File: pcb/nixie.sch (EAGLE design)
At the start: 158 parts, among them IC1 STM32F100CXC, IC12 MAX603, IC2 74141N, IC3 DS3234, IC4 MAX1771, IC6 74HCT164D, IC7 DS18B20, IC8 MAX603, Q1 BUZ11BH, Q9 BSS123, X2 MINI-USB_4P-85-32004-10X

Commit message: almost done
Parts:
- removed S6: (no value), SparkFun:TAC_SWITCHPTH
- added S1, S3: (no value), Mine:TAC_SWITCH
- C1, C10, C11, C12, C13, C14, C15, C18, C20, C21, C22, C25, C26, C27, C35, C36, C4, C52, C53, C7, C8, C9, C93: value (none) -> 100n
- C16, C17, C28, C29, C92: value (none) -> 10u
- C2, C23, C3, C34, C5, Q3, R12, R51, R9: value (none) -> nc
- C24: value (none) -> 100n; device rcl:C-EUC1206 -> rcl:C-EUC0603
- C50, C51: value (none) -> 1u
- C54, L1: value (none) -> 100u
- C6: value (none) -> 2.2u 250V
- D10, D11, D8, D9: value CGRM4001-G -> (none); device diode:CGRM4001-G -> diode:DIODE-SOD123
- D2, D3, D4, D5, D6, D7: value CGRM4001-G -> 1n4148
- R1, R36, R37, R50, R6: value (none) -> 10k
- R13, R8: value (none) -> 22k
- R14, R16, R18, R20, R22, R24: value (none) -> 1M
- R15, R17, R19, R21, R23, R25: value (none) -> 47k
- R2: value (none) -> 100
- R3: value (none) -> 1k
- R30, R31: value (none) -> tbc
- R38: value (none) -> 220k
- R39, R40, R41: value (none) -> 200k
- R4: value (none) -> 0.05
- R5: value (none) -> 1M5
- R7: value (none) -> 4k7 trim
- S2, S4, S5: device SparkFun:TAC_SWITCHPTH -> Mine:TAC_SWITCH
- T1, T11, T13, T14, T3, T5, T7, T9: value (none) -> pnphv
- T10, T12, T2, T4, T6, T8: value (none) -> npnhvsmd
- T21, T22: value (none) -> npnhvth
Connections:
- net +3V3: now also S3.1; no longer S2.2, S4.2, S5.2, S6.1, S6.2
- net BUT0: now also S5.2; no longer S5.3, S5.4
- net BUT1: now also S2.2; no longer S6.3, S6.4
- net BUT2: now also S4.2; no longer S4.3, S4.4
- net BUT3: now also S3.2; no longer S2.3, S2.4
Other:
- note added: "nc"
- note added: "tbc"

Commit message: deleted stuff for merging
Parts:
- removed C23: nc, rcl:C-EUC0603
- removed C93: 100n, rcl:C-EUC0603
- removed L2: (no value), wuerth-elektronik:WE-CBF_0805
- removed R9: nc, rcl:R-EU_R0805
- removed S1: (no value), Mine:TAC_SWITCH
- removed SV6: (no value), Mine:FE06-1ED
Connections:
- removed net RXD: SV6.2
- removed net TXD: SV6.3
- net GND: no longer C93.1
- net VBAT: no longer C93.2
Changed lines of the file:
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@@
 <part name="Q3" library="crystal" deviceset="CRYSTAL" device="CTS406" value="nc"/>
 <part name="SV4" library="Mine" deviceset="FE05-2W" device="ED"/>
-<part name="SV6" library="Mine" deviceset="FE06-1" device="ED"/>
 <part name="IC12" library="Mine" deviceset="MAX603" device=""/>
 <part name="C28" library="rcl" deviceset="C-EU" device="C0603" value="10u"/>
@@
 <part name="D8" library="diode" deviceset="DIODE-" device="SOD123"/>
 <part name="D9" library="diode" deviceset="DIODE-" device="SOD123"/>
-<part name="L2" library="wuerth-elektronik" deviceset="WE-CBF" device="_0805"/>
 <part name="C34" library="rcl" deviceset="CPOL-EU" device="SMCC" value="nc"/>
 <part name="GND9" library="supply1" deviceset="GND" device=""/>
@@
 <part name="R1" library="rcl" deviceset="R-EU_" device="R0603" value="10k"/>
 <part name="SJ2" library="SparkFun" deviceset="SOLDERJUMPER" device="NO"/>
-<part name="C23" library="rcl" deviceset="C-EU" device="C0603" value="nc"/>
-<part name="R9" library="rcl" deviceset="R-EU_" device="R0805" value="nc"/>
 <part name="+3V10" library="supply1" deviceset="+3V3" device=""/>
 <part name="+3V11" library="supply1" deviceset="+3V3" device=""/>
@@
 <part name="R51" library="rcl" deviceset="R-EU_" device="R0603" value="nc"/>
 <part name="C92" library="rcl" deviceset="C-EU" device="C0603" value="10u"/>
-<part name="C93" library="rcl" deviceset="C-EU" device="C0603" value="100n"/>
 <part name="GND13" library="supply1" deviceset="GND" device=""/>
 <part name="SJ3" library="SparkFun" deviceset="SOLDERJUMPER" device="NO"/>
@@
 <part name="R12" library="rcl" deviceset="R-EU_" device="R0603" value="nc"/>
 <part name="P+1" library="supply1" deviceset="+5V" device=""/>
-<part name="S1" library="Mine" deviceset="TAC_SWITCH" device=""/>
 <part name="S2" library="Mine" deviceset="TAC_SWITCH" device=""/>
 <part name="S3" library="Mine" deviceset="TAC_SWITCH" device=""/>
@@
 <instance part="Q3" gate="G$1" x="25.4" y="-5.08" rot="R90"/>
 <instance part="SV4" gate="G$1" x="266.7" y="-27.94"/>
-<instance part="SV6" gate="G$1" x="287.02" y="-27.94"/>
 <instance part="IC12" gate="G$1" x="-40.64" y="147.32"/>
 <instance part="C28" gate="G$1" x="-55.88" y="139.7"/>
@@
 <instance part="D8" gate="G$1" x="-71.12" y="205.74"/>
 <instance part="D9" gate="G$1" x="-73.66" y="182.88"/>
-<instance part="L2" gate="G$1" x="-76.2" y="226.06" rot="R90"/>
 <instance part="C34" gate="G$1" x="-43.18" y="210.82"/>
 <instance part="GND9" gate="1" x="-43.18" y="203.2"/>
@@
 <instance part="R1" gate="G$1" x="-91.44" y="38.1"/>
 <instance part="SJ2" gate="1" x="137.16" y="-35.56"/>
-<instance part="C23" gate="G$1" x="-162.56" y="43.18" rot="R90"/>
-<instance part="R9" gate="G$1" x="-154.94" y="50.8" rot="R270"/>
 <instance part="+3V10" gate="G$1" x="-154.94" y="60.96"/>
 <instance part="+3V11" gate="G$1" x="93.98" y="-22.86"/>
@@
 <instance part="R51" gate="G$1" x="20.32" y="-7.62"/>
 <instance part="C92" gate="G$1" x="-104.14" y="17.78"/>
-<instance part="C93" gate="G$1" x="-96.52" y="68.58"/>
 <instance part="GND13" gate="1" x="-96.52" y="73.66" rot="R180"/>
 <instance part="SJ3" gate="1" x="-104.14" y="63.5"/>
@@
 <instance part="R12" gate="G$1" x="48.26" y="106.68" rot="R90"/>
 <instance part="P+1" gate="1" x="48.26" y="114.3"/>
-<instance part="S1" gate="S" x="-10.16" y="-27.94" rot="R270"/>
 <instance part="S2" gate="S" x="2.54" y="-27.94" rot="R270"/>
 <instance part="S3" gate="S" x="15.24" y="-27.94" rot="R270"/>
@@
 <wire x1="30.48" y1="48.26" x2="33.02" y2="48.26" width="0.1524" layer="91"/>
 </segment>
-<segment>
-<pinref part="C93" gate="G$1" pin="1"/>
-<pinref part="GND13" gate="1" pin="GND"/>
-</segment>
 </net>
 <net name="+5V" class="0">
@@
 <segment>
 <wire x1="294.64" y1="-30.48" x2="299.72" y2="-30.48" width="0.1524" layer="91"/>
-<pinref part="SV6" gate="G$1" pin="2"/>
 </segment>
 </net>
@@
 <segment>
 <wire x1="294.64" y1="-27.94" x2="299.72" y2="-27.94" width="0.1524" layer="91"/>
-<pinref part="SV6" gate="G$1" pin="3"/>
 </segment>
 </net>
@@
 <net name="VBAT" class="0">
 <segment>
-<wire x1="-86.36" y1="63.5" x2="-96.52" y2="63.5" width="0.1524" layer="91"/>
+<wire x1="-86.36" y1="63.5" x2="-99.06" y2="63.5" width="0.1524" layer="91"/>
 <label x="-93.98" y="63.5" size="1.778" layer="95"/>
 <pinref part="IC1" gate="G$1" pin="VBAT"/>
-<pinref part="C93" gate="G$1" pin="2"/>
-<wire x1="-96.52" y1="63.5" x2="-99.06" y2="63.5" width="0.1524" layer="91"/>
-<junction x="-96.52" y="63.5"/>
 <pinref part="SJ3" gate="1" pin="2"/>
 </segment>

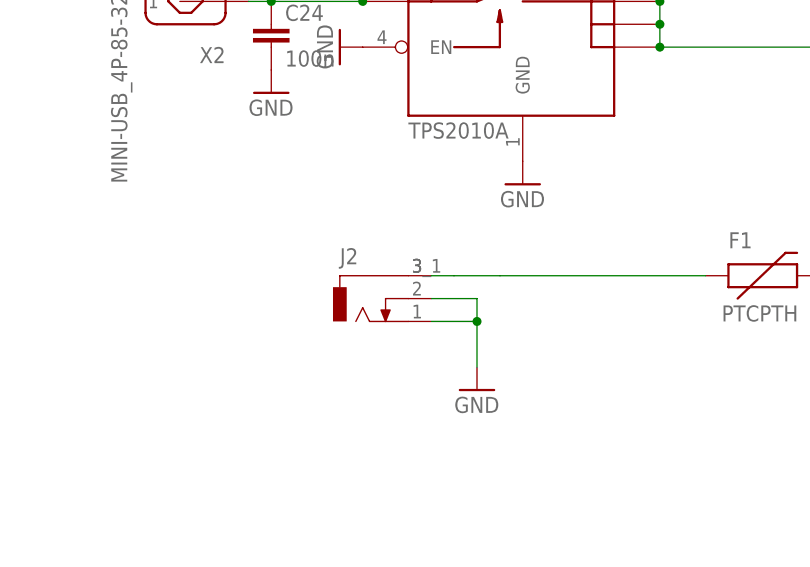
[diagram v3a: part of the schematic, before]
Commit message: off for fab
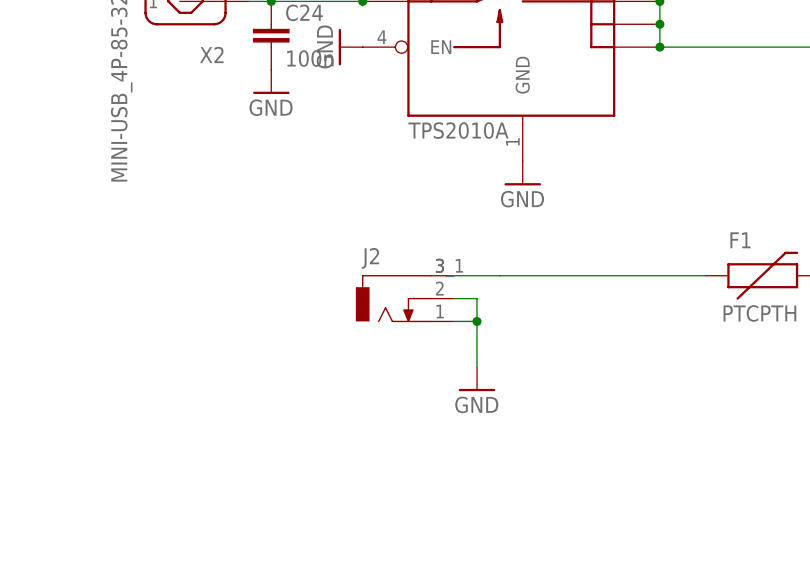
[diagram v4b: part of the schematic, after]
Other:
- moved on the sheet: J2
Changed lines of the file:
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@@
 <instance part="SV1" gate="G$1" x="320.04" y="137.16"/>
 <instance part="SV2" gate="G$1" x="215.9" y="76.2"/>
-<instance part="J2" gate="G$1" x="-129.54" y="180.34"/>
+<instance part="J2" gate="G$1" x="-127" y="180.34"/>
 <instance part="C22" gate="G$1" x="-5.08" y="182.88"/>
 <instance part="Q3" gate="G$1" x="25.4" y="-5.08" rot="R90"/>
@@
 <segment>
 <wire x1="-116.84" y1="177.8" x2="-116.84" y2="172.72" width="0.1524" layer="91"/>
-<wire x1="-121.92" y1="180.34" x2="-116.84" y2="180.34" width="0.1524" layer="91"/>
+<wire x1="-119.38" y1="180.34" x2="-116.84" y2="180.34" width="0.1524" layer="91"/>
 <wire x1="-116.84" y1="180.34" x2="-116.84" y2="177.8" width="0.1524" layer="91"/>
-<wire x1="-116.84" y1="177.8" x2="-121.92" y2="177.8" width="0.1524" layer="91"/>
+<wire x1="-116.84" y1="177.8" x2="-119.38" y2="177.8" width="0.1524" layer="91"/>
 <junction x="-116.84" y="177.8"/>
 <pinref part="GND30" gate="1" pin="GND"/>
@@
 <pinref part="J2" gate="G$1" pin="4"/>
 <wire x1="-114.3" y1="182.88" x2="-91.44" y2="182.88" width="0.1524" layer="91"/>
-<wire x1="-119.38" y1="182.88" x2="-121.92" y2="182.88" width="0.1524" layer="91"/>
-</segment>
-</net>
+</segment>
+</net>
